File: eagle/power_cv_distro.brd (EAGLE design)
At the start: 100.6 x 80.6 mm, 20 parts, among them U1 POWER, U2 POWER, U3 POWER, U5 POWER, U6 POWER, U7 POWER, U9 POWER

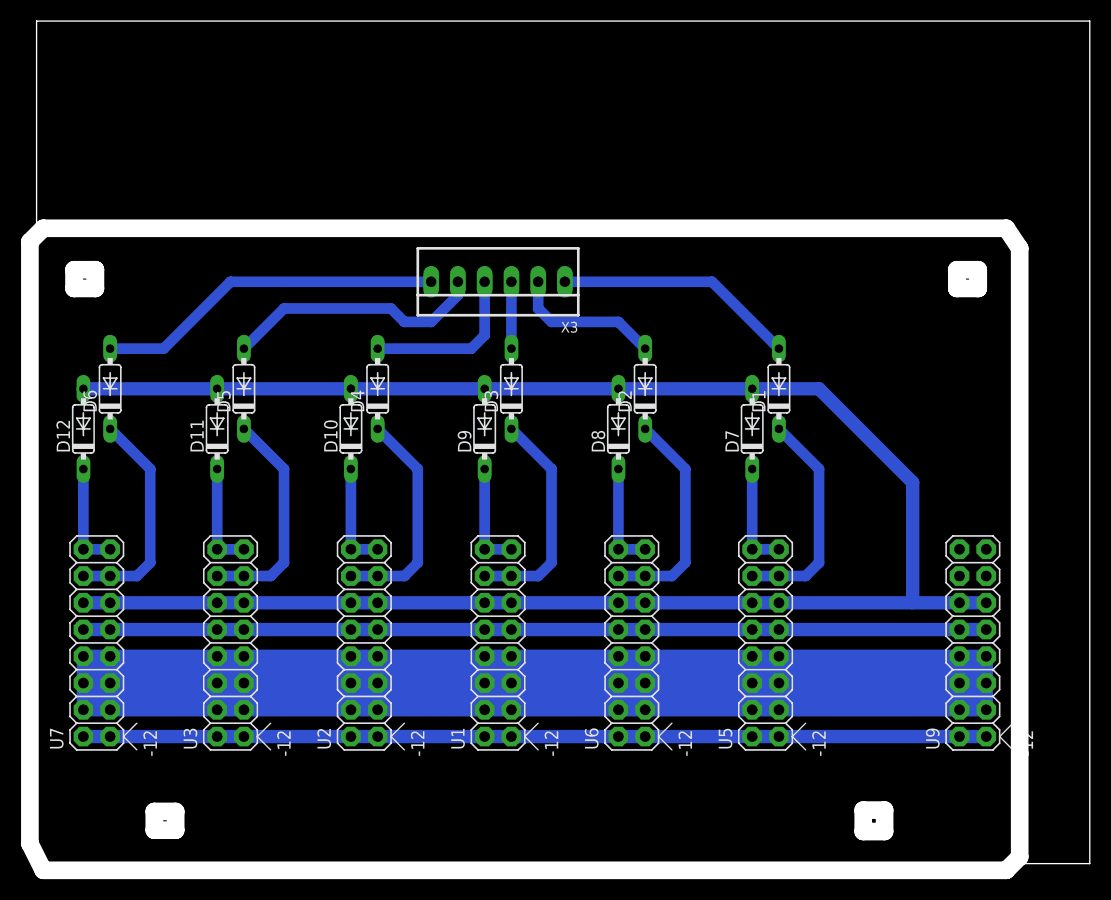
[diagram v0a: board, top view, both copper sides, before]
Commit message: added layout png
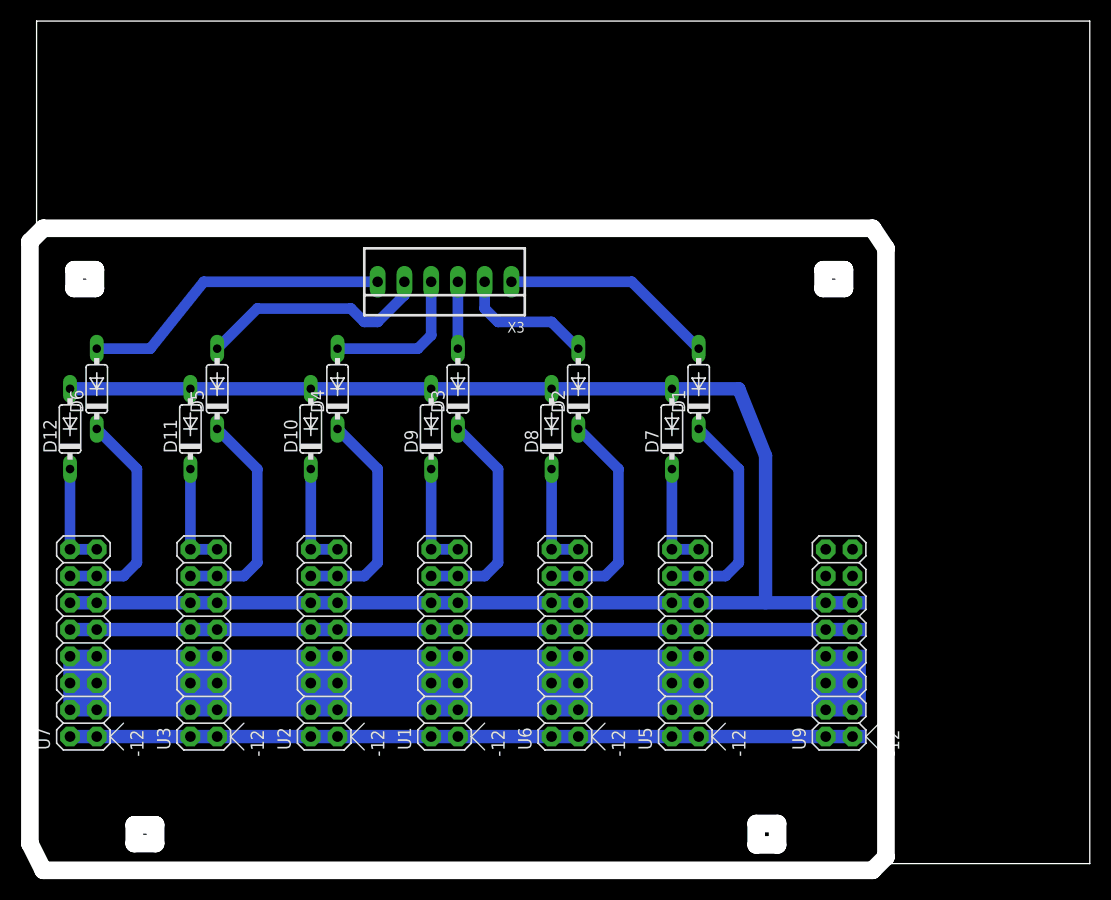
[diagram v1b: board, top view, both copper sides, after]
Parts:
- moved U9 12.7 mm to (76.2, 18.4)
- moved U5 7.62 mm to (61.6, 18.4)
- moved D1 7.62 mm to (62.9, 45.1)
- moved D7 7.62 mm to (60.3, 41.3)
- moved U6 6.35 mm to (50.2, 18.4)
- moved D2 6.35 mm to (51.4, 45.1)
- moved D8 6.35 mm to (48.9, 41.3)
- moved D3 5.08 mm to (40.0, 45.1)
- moved D9 5.08 mm to (37.5, 41.3)
- moved U1 5.08 mm to (38.7, 18.4)
- moved X3 5.08 mm to (38.7, 55.2)
- moved D10 3.81 mm to (26.0, 41.3)
- moved D4 3.81 mm to (28.6, 45.1)
- moved U2 3.81 mm to (27.3, 18.4)
- moved D11 2.54 mm to (14.6, 41.3)
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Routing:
- net +5V: track 98.3 -> 90.0 mm
- net N$6: track 33.1 -> 29.7 mm
- net N$5: track 24.7 -> 22.2 mm
- net N$1: track 23.0 -> 20.4 mm
- net N$4: track 15.8 -> 14.5 mm
- net N$2: track 14.3 -> 13.0 mm
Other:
- outline, holes or cut-outs redrawn
